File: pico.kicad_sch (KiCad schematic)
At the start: 7 parts, among them J12 I2C, Q4 DMG2305UX, U14 Pico

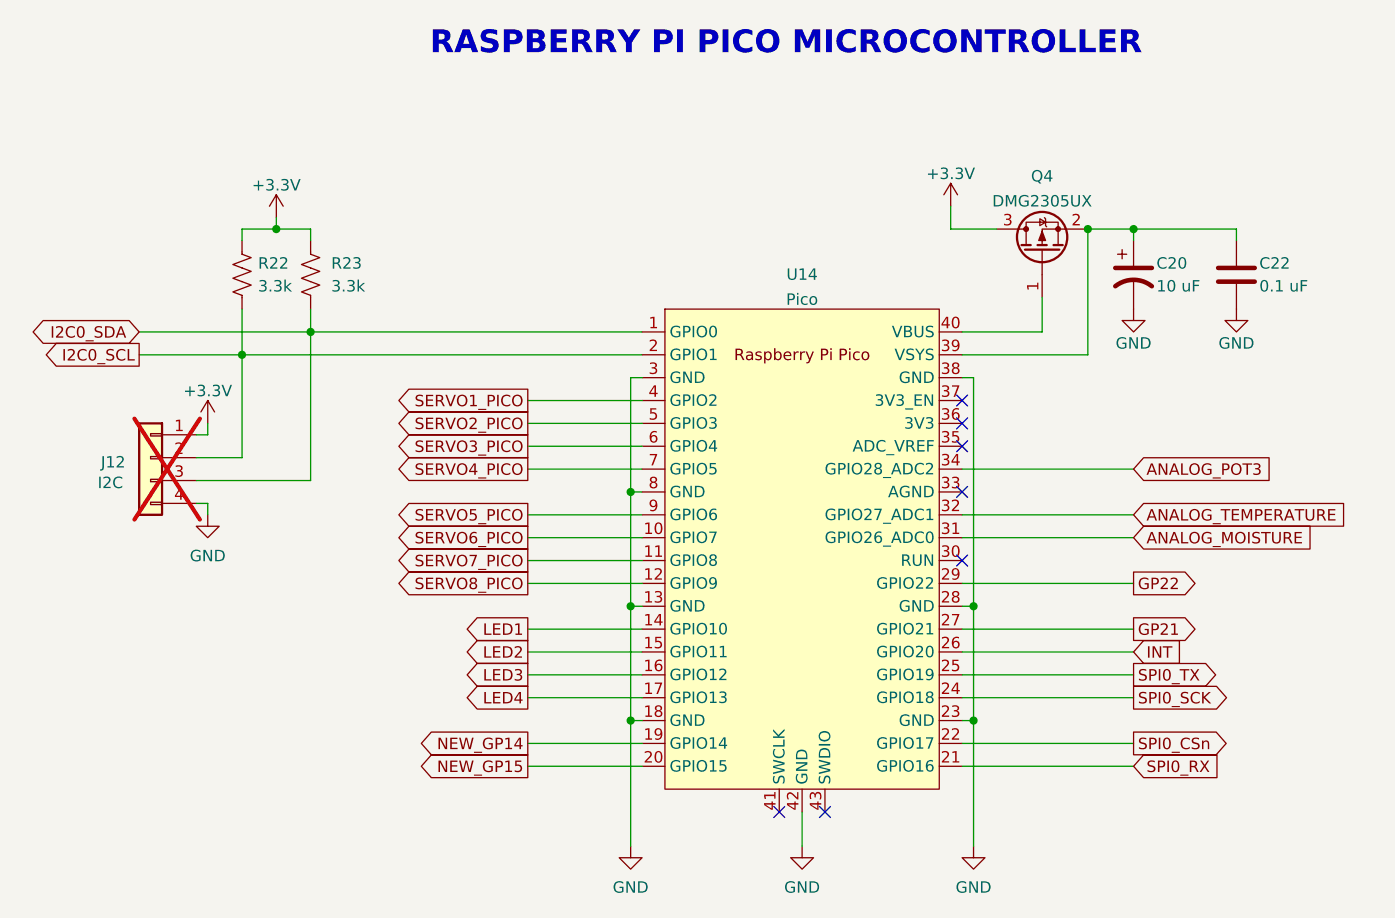
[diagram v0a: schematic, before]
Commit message: more cleanup and added notes for review
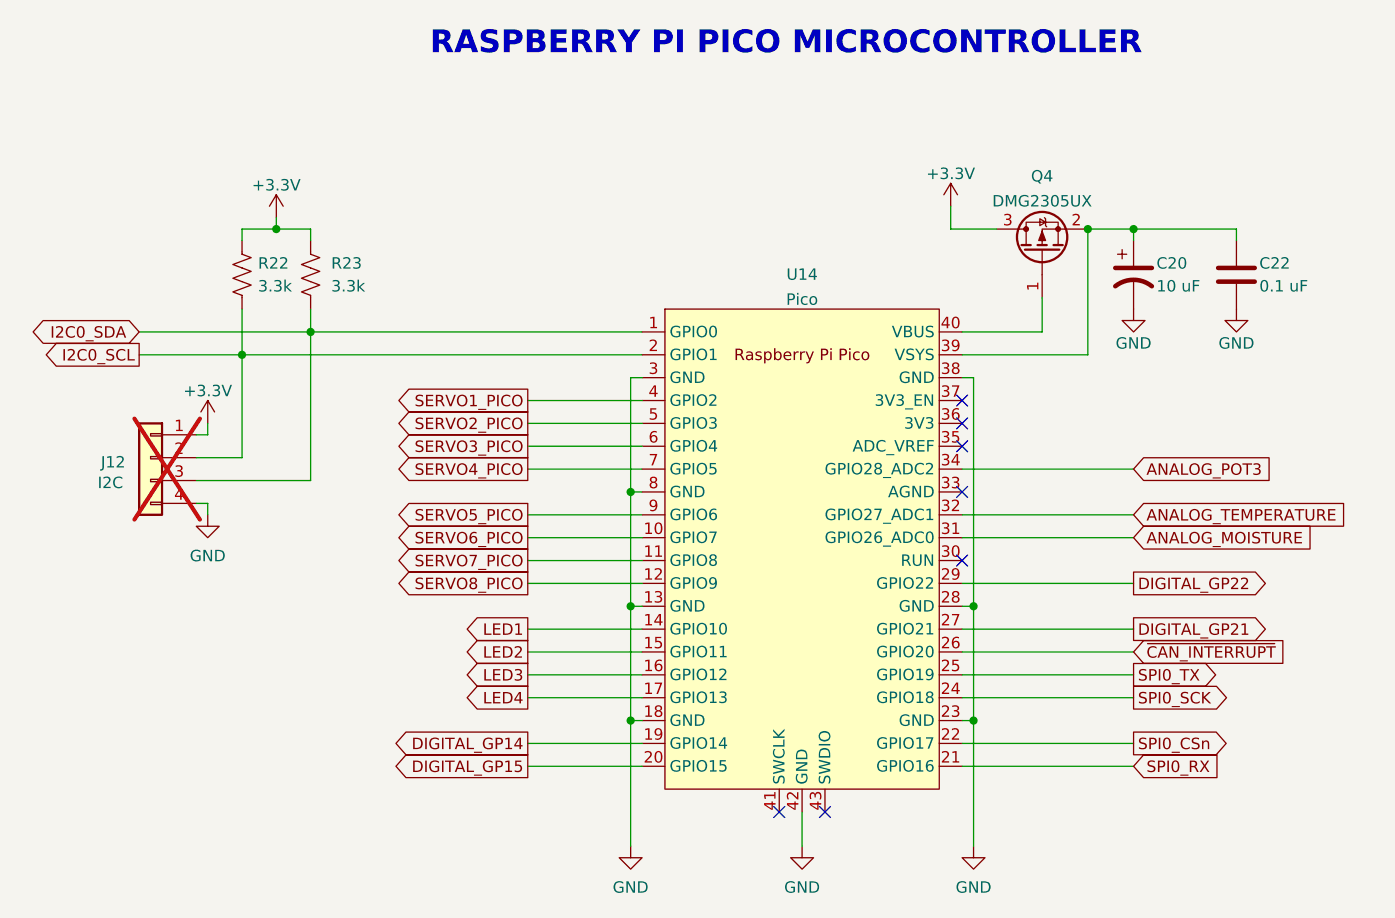
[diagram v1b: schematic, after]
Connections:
- net GP21 renamed DIGITAL_GP21
- net GP22 renamed DIGITAL_GP22
- net INT renamed ~{CAN_INTERRUPT}
- net NEW_GP14 renamed DIGITAL_GP14
- net NEW_GP15 renamed DIGITAL_GP15
